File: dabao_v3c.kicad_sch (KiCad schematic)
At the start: 61 parts, among them J1 USB_C_Receptacle_USB2.0_16P, Q1 LP0404N3T5G, Q2 LN237N3T5G, SW1 SKTAAAE010, SW2 SKTAAAE010, U1 baochip1x, U3 SMD IC PMIC;DCDC Buck-ADJ-1A,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, U4 XIAO-HALF-HOLE-23P, U5 EMS4000RSW, U7 SGM40567-4.2XG/TR, U8 SX1801CCR, U9 SMD IC PMIC;DCDC Buck-ADJ-1A,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, Y2 48.000MHz

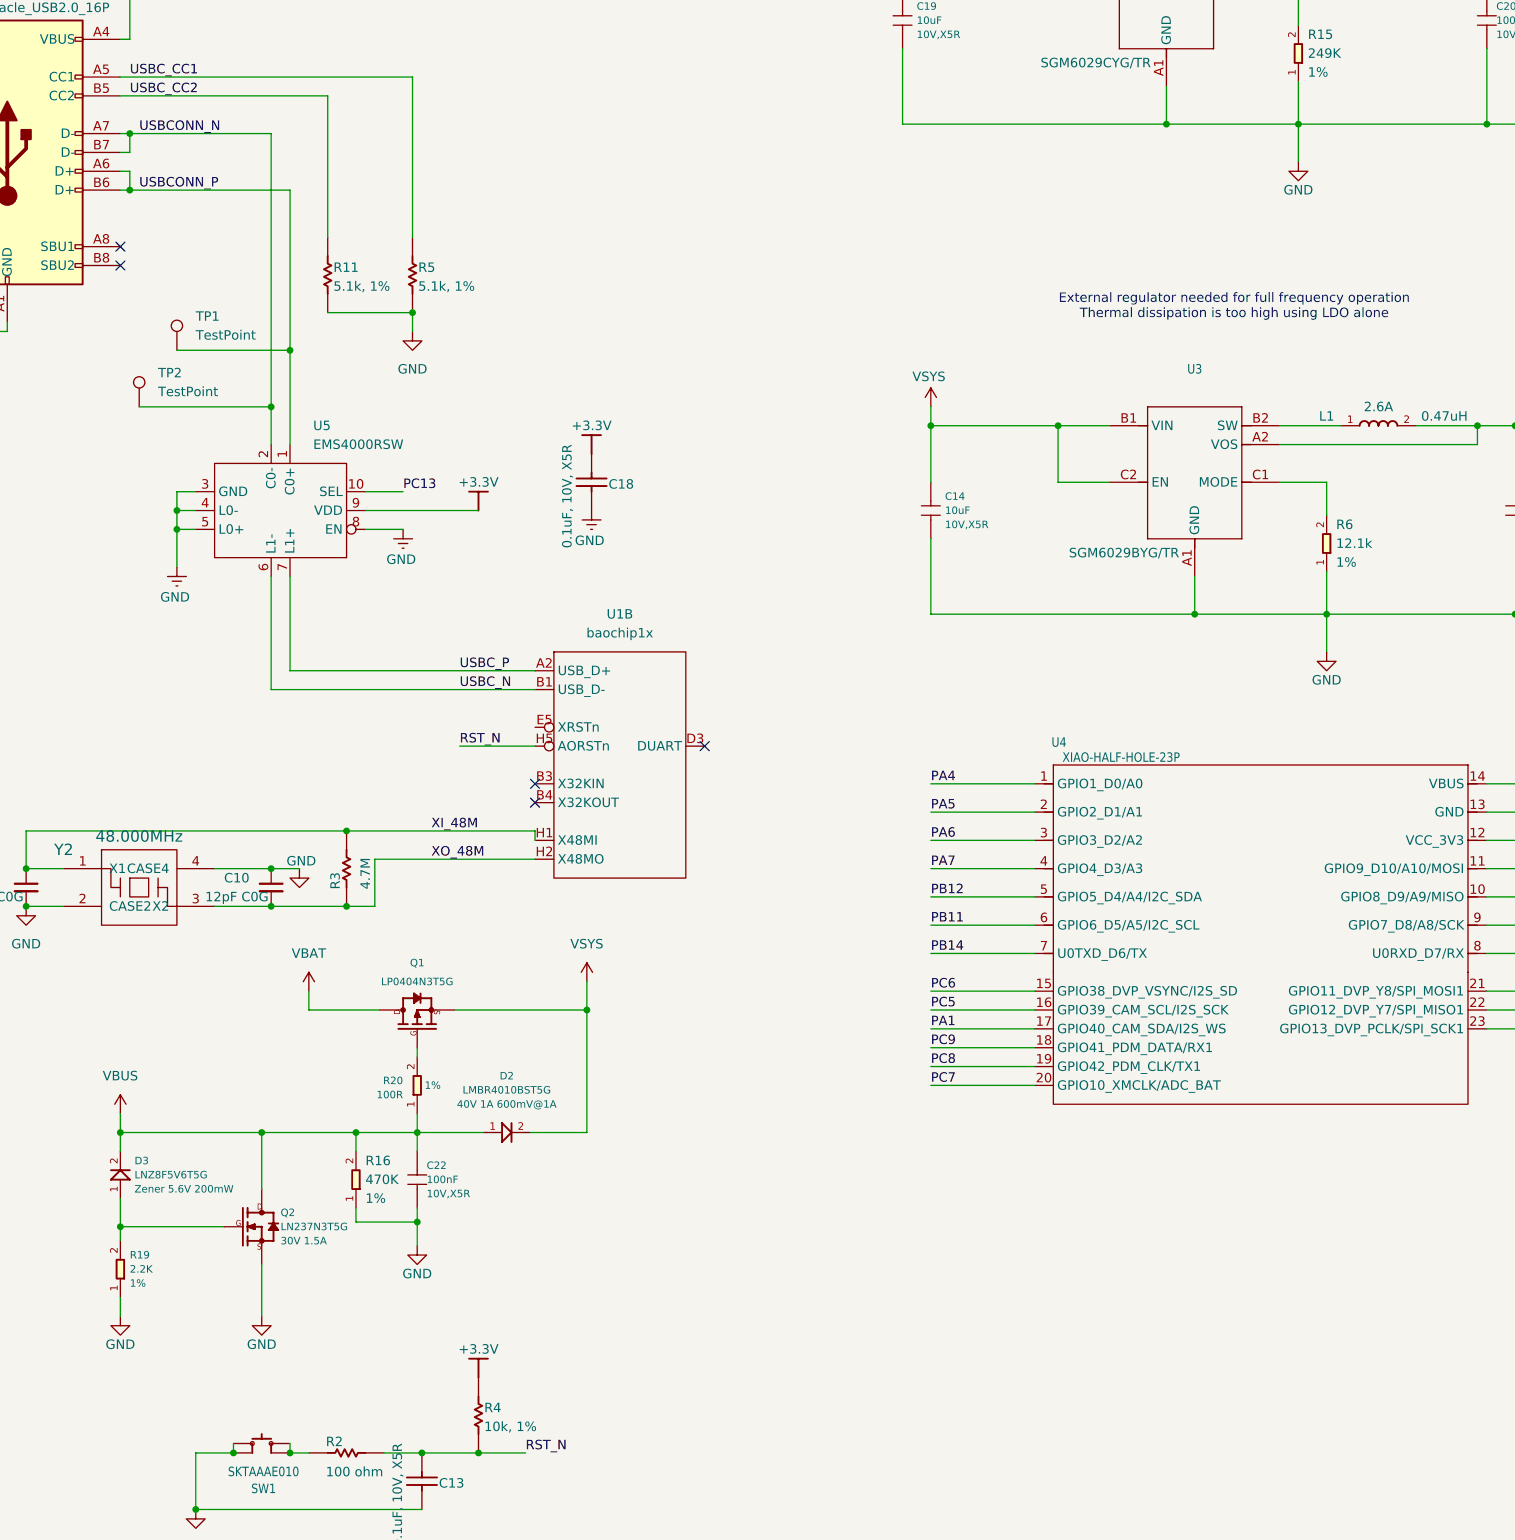
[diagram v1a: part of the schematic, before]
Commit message: now with more pins
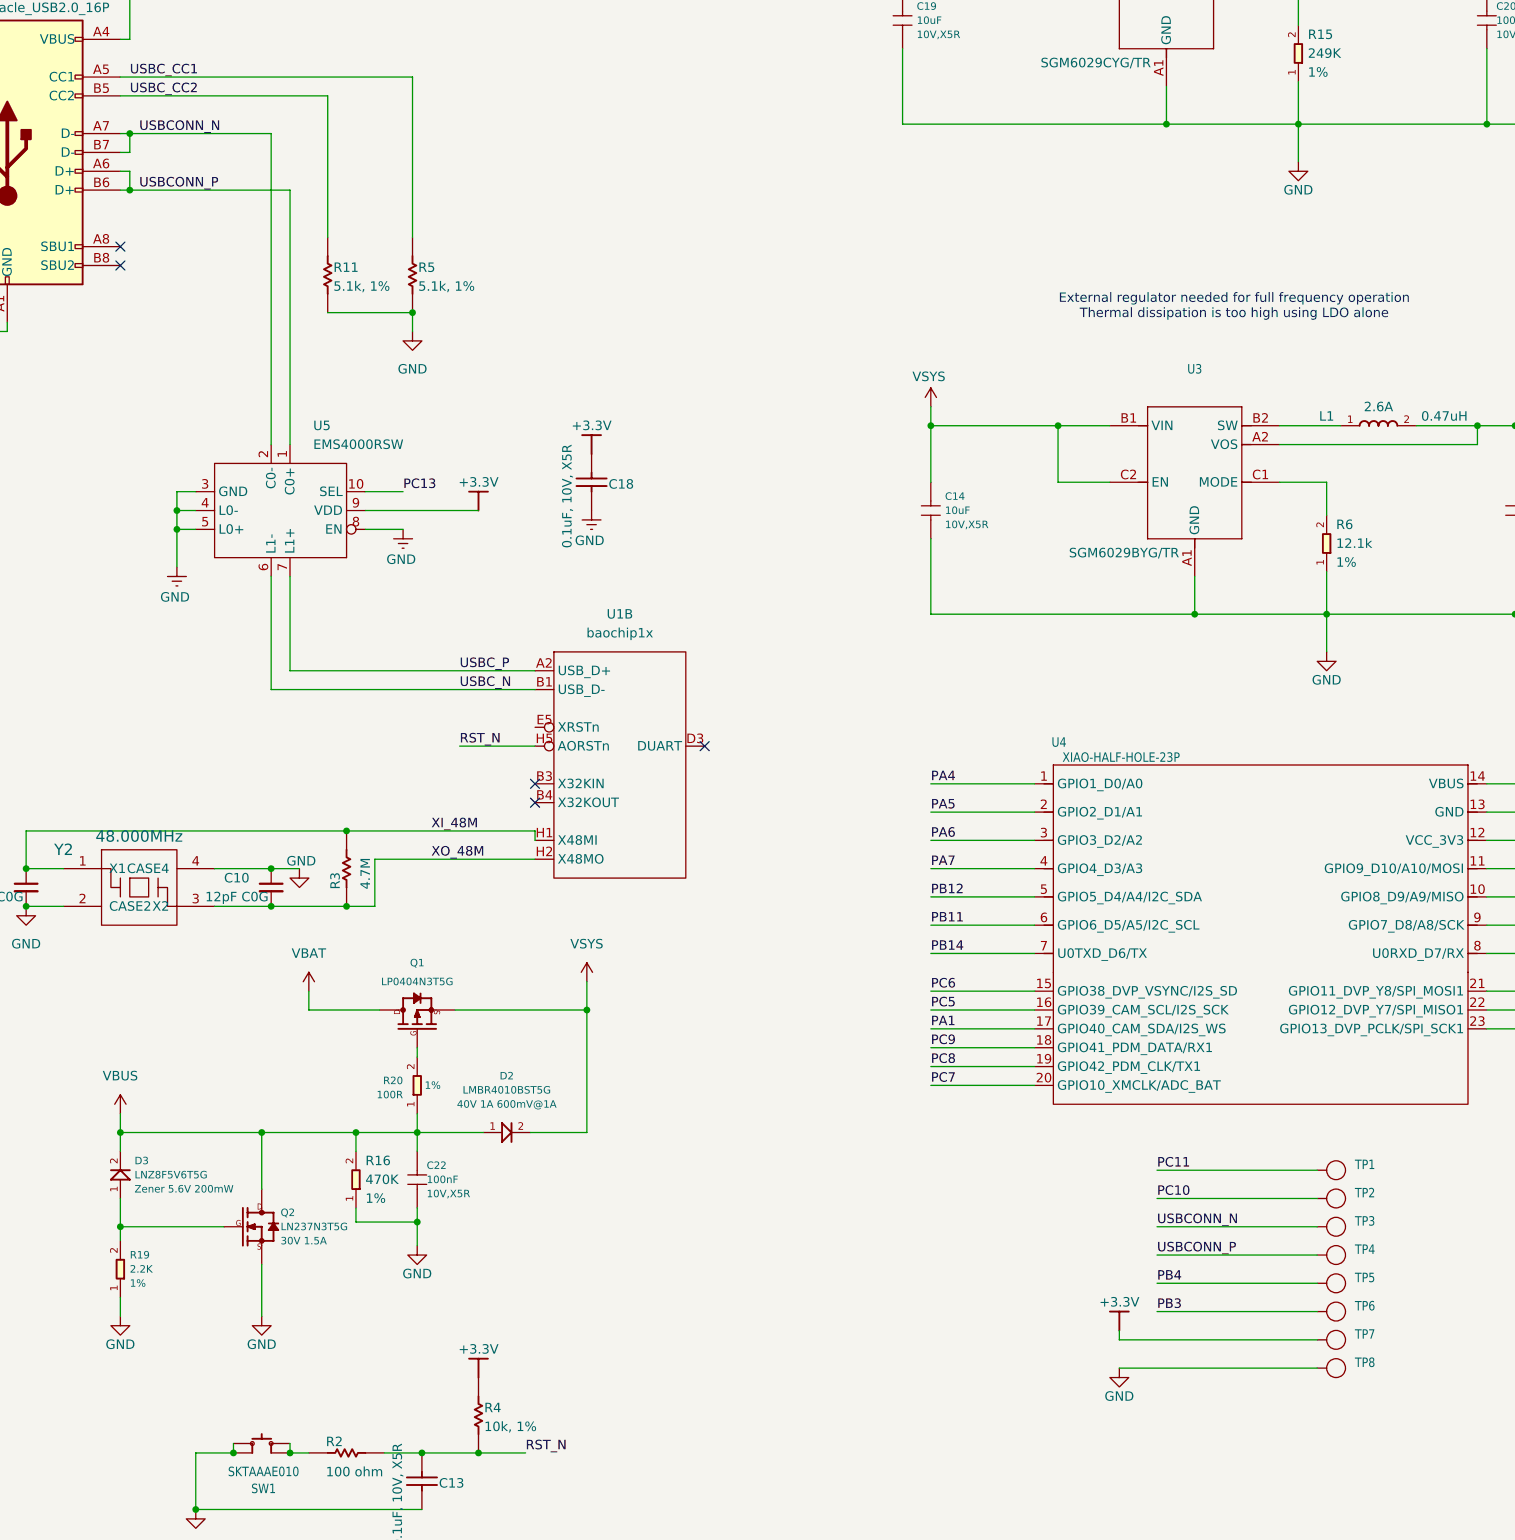
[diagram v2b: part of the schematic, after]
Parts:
- removed TP1, TP2: TestPoint, TestPoint:TestPoint_Pad_D1.0mm, symbol Connector:TestPoint
- added TP1, TP2, TP3, TP4, TP5, TP6, TP7, TP8: TEST-POINT'4545', xiao:TP-D45MIL, symbol XIAO ESP32S3_v1.2_230725-eagle-import:TEST-POINT'4545'
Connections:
- net +3.3V: now also TP7.T
- net GND: now also TP8.T
- net PB3: now also TP6.T
- net PB4: now also TP5.T
- net PC10: now also TP2.T
- net PC11: now also TP1.T
- net USBCONN_N: now also TP3.T
- net USBCONN_P: now also TP4.T
